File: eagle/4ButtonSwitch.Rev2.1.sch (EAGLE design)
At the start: 44 parts

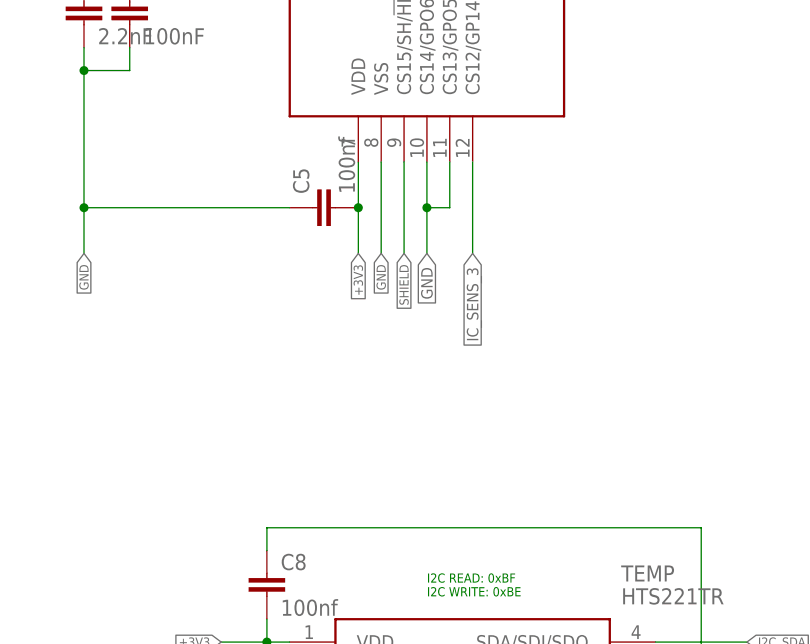
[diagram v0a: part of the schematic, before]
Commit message: Rev 2.1
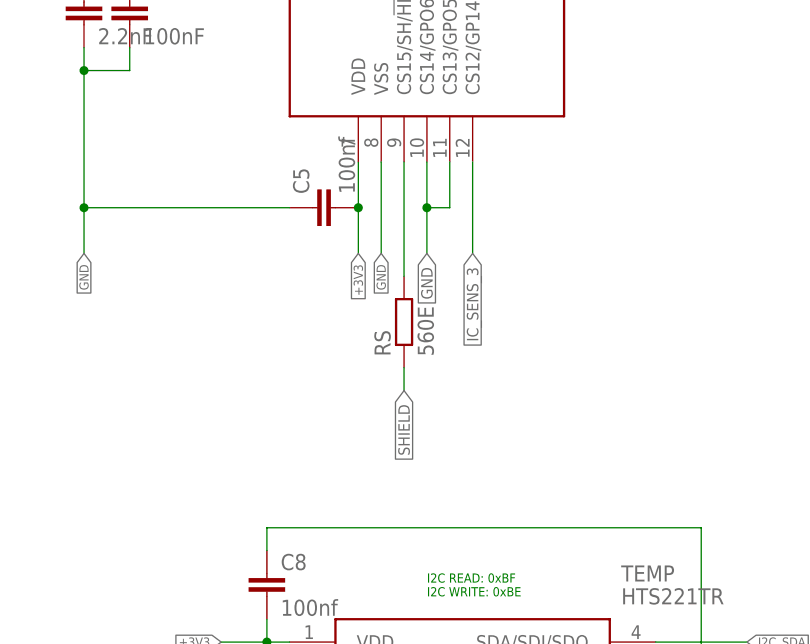
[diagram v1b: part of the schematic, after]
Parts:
- added RS: 560E, resistor:R-EU_R0402
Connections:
- new net N$1: RS.2, SENSORMCU.CS15/SH/!HI
- net SHIELD: now also RS.1; no longer SENSORMCU.CS15/SH/!HI
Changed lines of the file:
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@@
 <part name="C11" library="rcl" library_urn="urn:adsk.eagle:library:334" deviceset="C-EU" device="C0402" package3d_urn="urn:adsk.eagle:package:23626/1" value="4.7uf"/>
 <part name="S1" library="PCM12SMTR" deviceset="PCM12SMTR" device=""/>
+<part name="RS" library="resistor" library_urn="urn:adsk.eagle:library:348" deviceset="R-EU_" device="R0402" package3d_urn="urn:adsk.eagle:package:26058/1" value="560E"/>
 </parts>
 <sheets>
@@
 <instance part="C11" gate="G$1" x="109.22" y="17.78"/>
 <instance part="S1" gate="G$1" x="345.44" y="-35.56"/>
+<instance part="RS" gate="G$1" x="274.32" y="-30.48" rot="R90"/>
 </instances>
 <busses>
@@
 <net name="SHIELD" class="0">
 <segment>
-<pinref part="SENSORMCU" gate="G$1" pin="CS15/SH/!HI"/>
-<wire x1="274.32" y1="-12.7" x2="274.32" y2="-22.86" width="0.1524" layer="91"/>
-<label x="274.32" y="-22.86" size="1.016" layer="95" rot="R270" xref="yes"/>
-</segment>
-<segment>
 <pinref part="S1" gate="G$1" pin="3"/>
 <wire x1="365.76" y1="-35.56" x2="375.92" y2="-35.56" width="0.1524" layer="91"/>
 <label x="375.92" y="-35.56" size="1.27" layer="95" xref="yes"/>
 </segment>
+<segment>
+<pinref part="RS" gate="G$1" pin="1"/>
+<wire x1="274.32" y1="-35.56" x2="274.32" y2="-38.1" width="0.1524" layer="91"/>
+<label x="274.32" y="-38.1" size="1.27" layer="95" rot="R270" xref="yes"/>
+</segment>
 </net>
 <net name="USART2_TX" class="0">
@@
 </segment>
 </net>
+<net name="N$1" class="0">
+<segment>
+<pinref part="SENSORMCU" gate="G$1" pin="CS15/SH/!HI"/>
+<wire x1="274.32" y1="-12.7" x2="274.32" y2="-25.4" width="0.1524" layer="91"/>
+<pinref part="RS" gate="G$1" pin="2"/>
+</segment>
+</net>
